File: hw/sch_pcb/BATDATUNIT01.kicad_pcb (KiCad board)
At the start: 2 copper layers, 136.2 x 85.9 mm, 221 parts, among them J1 USBC_USB4105-GF-A, J2 SD_Card-FPS009-4200-0, J3 HEADER_2x03, J4 46436-9327, Q1 BC817-25, Q2 BC817-25, Q3 BC817-25, Q4 BC817-25, Q5 BC817-25, Q6 BC817-25, Q7 BSS83P, SW1 SKRTLAE010, SW2 KMT031, SW3 SKRTLAE010, SW4 KMT031, U1 MAX14502AETL+, U10 PCF85263A, U11 TCA4307, U12 BQ34Z100, U13 BQ25628E, U14 SN74HC164P, U15 TPS631000DRLR, U16 TPS631000DRLR, U17 TPS631000DRLR, U18 TPS22965-Q1, U2 USBLC6-2SC6, U4 PCA9541ABS/01, U5 AT24CS64-SSHM, U6 SHT35-DIS, U7 TMUX1574DYYR, U8 ATMEGA1284P-AU, U9 MS561101BA03-50, Y1 19.2 MHz, Y2 8 MHz, Y3 ABS07-120-32.768KHZ-T

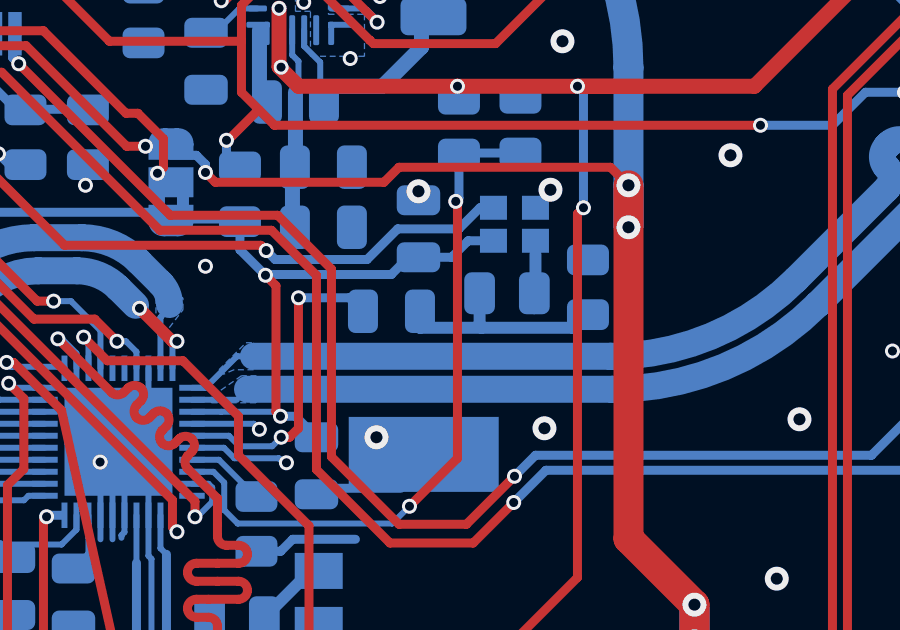
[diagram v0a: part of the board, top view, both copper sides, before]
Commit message: Change oscillator footprint. WIP
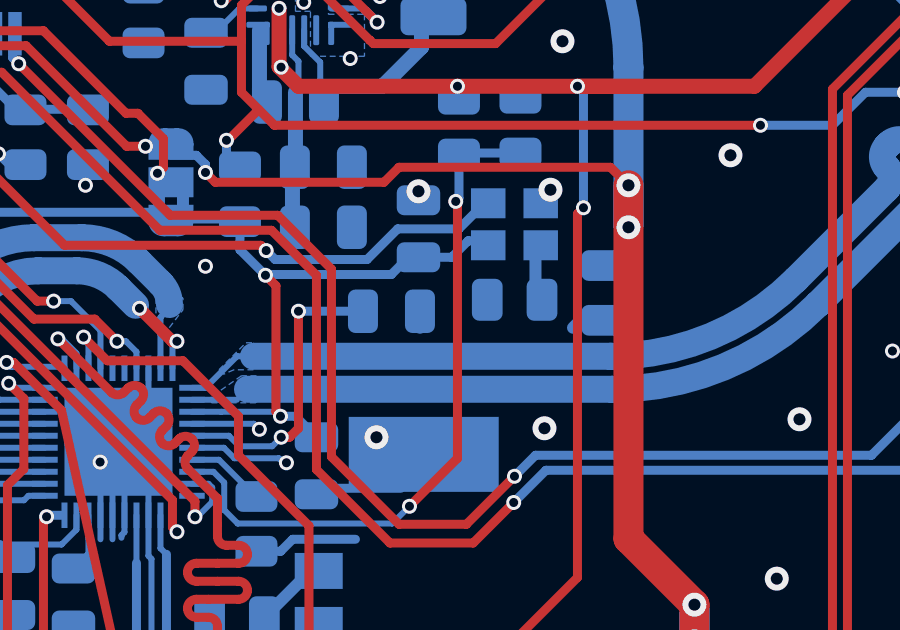
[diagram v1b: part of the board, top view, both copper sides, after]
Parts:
- Y1: footprint Crystal:Crystal_SMD_2016-4Pin_2.0x1.6mm -> Crystal:Crystal_SMD_2520-4Pin_2.5x2.0mm
- moved R4 0.51 mm to (189.0, 94.5)
- moved R3 0.34 mm to (186.1, 94.7)
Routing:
- net Net-(C49-Pad1): track 7.74 -> 1.91 mm
- net /FREF: track 10.6 -> 10.00 mm
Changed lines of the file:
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@@
   )
   (footprint "Resistor_SMD:R_0805_2012Metric" (layer "B.Cu")
-    (at 188.55 94.3 90)
+    (at 189.0268 94.488 90)
     (descr "Resistor SMD 0805 (2012 Metric), square (rectangular) end terminal, IPC_7351 nominal, (Body size source: IPC-SM-782 page 72, https://www.pcb-3d.com/wordpress/wp-content/uploads/ipc-sm-782a_amendment_1_and_2.pdf), generated with kicad-footprint-generator")
     (tags "resistor")
@@
   )
   (footprint "Resistor_SMD:R_0805_2012Metric" (layer "B.Cu")
-    (at 185.85 94.5 180)
+    (at 186.1058 94.7166 180)
     (descr "Resistor SMD 0805 (2012 Metric), square (rectangular) end terminal, IPC_7351 nominal, (Body size source: IPC-SM-782 page 72, https://www.pcb-3d.com/wordpress/wp-content/uploads/ipc-sm-782a_amendment_1_and_2.pdf), generated with kicad-footprint-generator")
     (tags "resistor")
@@
     )
   )
-  (footprint "Crystal:Crystal_SMD_2016-4Pin_2.0x1.6mm" (layer "B.Cu")
+  (footprint "Crystal:Crystal_SMD_2520-4Pin_2.5x2.0mm" (layer "B.Cu")
     (at 186.1 92.2)
-    (descr "SMD Crystal SERIES SMD2016/4 http://www.q-crystal.com/upload/5/2015552223166229.pdf, 2.0x1.6mm^2 package")
+    (descr "SMD Crystal SERIES SMD2520/4 http://www.newxtal.com/UploadFiles/Images/2012-11-12-09-29-09-776.pdf, 2.5x2.0mm^2 package")
     (tags "SMD SMT crystal")
     (property "Sheetfile" "BATDATUNIT01.kicad_sch")
@@
     (property "ki_keywords" "Crystal Clock Oscillator")
     (attr smd)
-    (fp_text reference "Y1" (at 2.05 -1.35) (layer "B.SilkS")
-        (effects (font (size 0.8 0.8) (thickness 0.1)) (justify mirror))
+    (fp_text reference "Y1" (at 0 2.2 180) (layer "B.SilkS")
+        (effects (font (size 1 1) (thickness 0.15)) (justify mirror))
     )
-    (fp_text value "19.2 MHz" (at 0 -2) (layer "B.Fab")
+    (fp_text value "19.2 MHz" (at 0 -2.2 180) (layer "B.Fab")
         (effects (font (size 1 1) (thickness 0.15)) (justify mirror))
     )
-    (fp_text user "${REFERENCE}" (at 0 0) (layer "B.Fab")
-        (effects (font (size 0.5 0.5) (thickness 0.075)) (justify mirror))
+    (fp_text user "${REFERENCE}" (at 0 0 180) (layer "B.Fab")
+        (effects (font (size 0.6 0.6) (thickness 0.09)) (justify mirror))
     )
-    (fp_line (start -1.35 -1.15) (end 1.35 -1.15)
+    (fp_line (start -1.65 -1.4) (end 1.65 -1.4)
       (stroke (width 0.12) (type solid)) (layer "B.SilkS"))
-    (fp_line (start -1.35 1.15) (end -1.35 -1.15)
+    (fp_line (start -1.65 1.4) (end -1.65 -1.4)
       (stroke (width 0.12) (type solid)) (layer "B.SilkS"))
-    (fp_line (start -1.4 -1.3) (end 1.4 -1.3)
+    (fp_line (start -1.7 -1.5) (end 1.7 -1.5)
       (stroke (width 0.05) (type solid)) (layer "B.CrtYd"))
-    (fp_line (start -1.4 1.3) (end -1.4 -1.3)
+    (fp_line (start -1.7 1.5) (end -1.7 -1.5)
       (stroke (width 0.05) (type solid)) (layer "B.CrtYd"))
-    (fp_line (start 1.4 -1.3) (end 1.4 1.3)
+    (fp_line (start 1.7 -1.5) (end 1.7 1.5)
       (stroke (width 0.05) (type solid)) (layer "B.CrtYd"))
-    (fp_line (start 1.4 1.3) (end -1.4 1.3)
+    (fp_line (start 1.7 1.5) (end -1.7 1.5)
       (stroke (width 0.05) (type solid)) (layer "B.CrtYd"))
-    (fp_line (start -1 -0.7) (end -1 0.7)
+    (fp_line (start -1.25 -0.9) (end -1.25 0.9)
       (stroke (width 0.1) (type solid)) (layer "B.Fab"))
-    (fp_line (start -1 -0.3) (end -0.5 -0.8)
+    (fp_line (start -1.25 0) (end -0.25 -1)
       (stroke (width 0.1) (type solid)) (layer "B.Fab"))
-    (fp_line (start -1 0.7) (end -0.9 0.8)
+    (fp_line (start -1.25 0.9) (end -1.15 1)
       (stroke (width 0.1) (type solid)) (layer "B.Fab"))
-    (fp_line (start -0.9 -0.8) (end -1 -0.7)
+    (fp_line (start -1.15 -1) (end -1.25 -0.9)
       (stroke (width 0.1) (type solid)) (layer "B.Fab"))
-    (fp_line (start -0.9 0.8) (end 0.9 0.8)
+    (fp_line (start -1.15 1) (end 1.15 1)
       (stroke (width 0.1) (type solid)) (layer "B.Fab"))
-    (fp_line (start 0.9 -0.8) (end -0.9 -0.8)
+    (fp_line (start 1.15 -1) (end -1.15 -1)
       (stroke (width 0.1) (type solid)) (layer "B.Fab"))
-    (fp_line (start 0.9 0.8) (end 1 0.7)
+    (fp_line (start 1.15 1) (end 1.25 0.9)
       (stroke (width 0.1) (type solid)) (layer "B.Fab"))
-    (fp_line (start 1 -0.7) (end 0.9 -0.8)
+    (fp_line (start 1.25 -0.9) (end 1.15 -1)
       (stroke (width 0.1) (type solid)) (layer "B.Fab"))
-    (fp_line (start 1 0.7) (end 1 -0.7)
+    (fp_line (start 1.25 0.9) (end 1.25 -0.9)
       (stroke (width 0.1) (type solid)) (layer "B.Fab"))
-    (pad "1" smd rect (at -0.7 -0.55) (size 0.9 0.8) (layers "B.Cu" "B.Paste" "B.Mask")
+    (pad "1" smd rect (at -0.875 -0.7) (size 1.15 1) (layers "B.Cu" "B.Paste" "B.Mask")
       (net 212 "/mode_osc") (pinfunction "EN") (pintype "input"))
-    (pad "2" smd rect (at 0.7 -0.55) (size 0.9 0.8) (layers "B.Cu" "B.Paste" "B.Mask")
+    (pad "2" smd rect (at 0.875 -0.7) (size 1.15 1) (layers "B.Cu" "B.Paste" "B.Mask")
       (net 1 "GND") (pinfunction "GND") (pintype "power_in"))
-    (pad "3" smd rect (at 0.7 0.55) (size 0.9 0.8) (layers "B.Cu" "B.Paste" "B.Mask")
+    (pad "3" smd rect (at 0.875 0.7) (size 1.15 1) (layers "B.Cu" "B.Paste" "B.Mask")
       (net 165 "Net-(Y1-OUT)") (pinfunction "OUT") (pintype "output"))
-    (pad "4" smd rect (at -0.7 0.55) (size 0.9 0.8) (layers "B.Cu" "B.Paste" "B.Mask")
+    (pad "4" smd rect (at -0.875 0.7) (size 1.15 1) (layers "B.Cu" "B.Paste" "B.Mask")
       (net 89 "+3.3V") (pinfunction "VDD") (pintype "power_in"))
-    (model "${KICAD7_3DMODEL_DIR}/Crystal.3dshapes/Crystal_SMD_MicroCrystal_CC8V-T1A-2Pin_2.0x1.2mm.step"
+    (model "${KICAD6_3DMODEL_DIR}/Crystal.3dshapes/Crystal_SMD_2520-4Pin_2.5x2.0mm.wrl"
       (offset (xyz 0 0 0))
       (scale (xyz 1 1 1))
@@
   (segment (start 186.8 93.2) (end 186.8 94.9625) (width 0.4) (layer "B.Cu") (net 165))
   (segment (start 186.8 94.9625) (end 186.7625 95) (width 0.4) (layer "B.Cu") (net 165))
-  (segment (start 178.9 99) (end 178.9 94.6505) (width 0.3) (layer "F.Cu") (net 166))
-  (segment (start 178.601527 99.298473) (end 178.9 99) (width 0.3) (layer "F.Cu") (net 166))
-  (segment (start 178.9 94.6505) (end 178.9005 94.65) (width 0.3) (layer "F.Cu") (net 166))
-  (segment (start 178.3255 99.298473) (end 178.601527 99.298473) (width 0.3) (layer "F.Cu") (net 166))
-  (via (at 178.9005 94.65) (size 0.5) (drill 0.3) (layers "F.Cu" "B.Cu") (net 166))
+  (segment (start 178.9 95.0976) (end 178.9 99) (width 0.3) (layer "F.Cu") (net 166))
+  (segment (start 178.601527 99.298473) (end 178.3255 99.298473) (width 0.3) (layer "F.Cu") (net 166))
+  (segment (start 178.9 99) (end 178.601527 99.298473) (width 0.3) (layer "F.Cu") (net 166))
+  (via (at 178.9 95.0976) (size 0.5) (drill 0.3) (layers "F.Cu" "B.Cu") (net 166))
   (via (at 178.3255 99.298473) (size 0.5) (drill 0.3) (layers "F.Cu" "B.Cu") (net 166))
   (segment (start 176.581371 99.25) (end 175.35 99.25) (width 0.2) (layer "B.Cu") (net 166))
   (segment (start 178.3255 99.298473) (end 178.024173 99.5998) (width 0.2) (layer "B.Cu") (net 166))
+  (segment (start 181.0476 95.0976) (end 181.05 95.1) (width 0.3) (layer "B.Cu") (net 166))
   (segment (start 178.024173 99.5998) (end 176.931172 99.5998) (width 0.2) (layer "B.Cu") (net 166))
   (segment (start 176.931172 99.5998) (end 176.581371 99.25) (width 0.2) (layer "B.Cu") (net 166))
-  (segment (start 178.9005 94.65) (end 180.6 94.65) (width 0.3) (layer "B.Cu") (net 166))
-  (segment (start 180.6 94.65) (end 181.05 95.1) (width 0.3) (layer "B.Cu") (net 166))
+  (segment (start 178.9 95.0976) (end 181.0476 95.0976) (width 0.3) (layer "B.Cu") (net 166))
   (segment (start 125.53 123.77) (end 125.5 123.8) (width 0.3) (layer "F.Cu") (net 167))
   (segment (start 126.590661 123.77) (end 125.53 123.77) (width 0.3) (layer "F.Cu") (net 167))
@@
   (segment (start 168.8 79.95) (end 168.8 79) (width 0.3) (layer "B.Cu") (net 216))
   (segment (start 168.799739 79.950261) (end 168.8 79.95) (width 0.3) (layer "B.Cu") (net 216))
-  (segment (start 184.9375 94.55) (end 184.9375 95.5875) (width 0.4) (layer "B.Cu") (net 217))
-  (segment (start 185 95.65) (end 182.95 95.65) (width 0.4) (layer "B.Cu") (net 217))
+  (segment (start 189.0268 95.4005) (end 188.2995 95.4005) (width 0.4) (layer "B.Cu") (net 217))
   (segment (start 183.15 94.9) (end 182.95 95.1) (width 0.4) (layer "B.Cu") (net 217))
-  (segment (start 188.55 95.2125) (end 188.4875 95.2125) (width 0.4) (layer "B.Cu") (net 217))
-  (segment (start 188.4875 95.2125) (end 188.05 95.65) (width 0.4) (layer "B.Cu") (net 217))
-  (segment (start 188.05 95.65) (end 185 95.65) (width 0.4) (layer "B.Cu") (net 217))
-  (segment (start 184.9375 95.5875) (end 185 95.65) (width 0.4) (layer "B.Cu") (net 217))
   (segment (start 182.95 95.65) (end 182.95 95.1) (width 0.4) (layer "B.Cu") (net 217))
+  (segment (start 188.2995 95.4005) (end 188.05 95.65) (width 0.4) (layer "B.Cu") (net 217))
   (zone (net 14) (net_name "+BATT") (layer "F.Cu") (name "BAT+") (hatch edge 0.5)
     (priority 5)
